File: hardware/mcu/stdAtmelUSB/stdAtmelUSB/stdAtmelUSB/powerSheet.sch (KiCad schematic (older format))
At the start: 22 parts, among them J1 Conn_01x03_Male, U1 LTC3406ES5, U2 MAX40200AUK, U3 LTC3406ES5, U4 MAX40200AUK

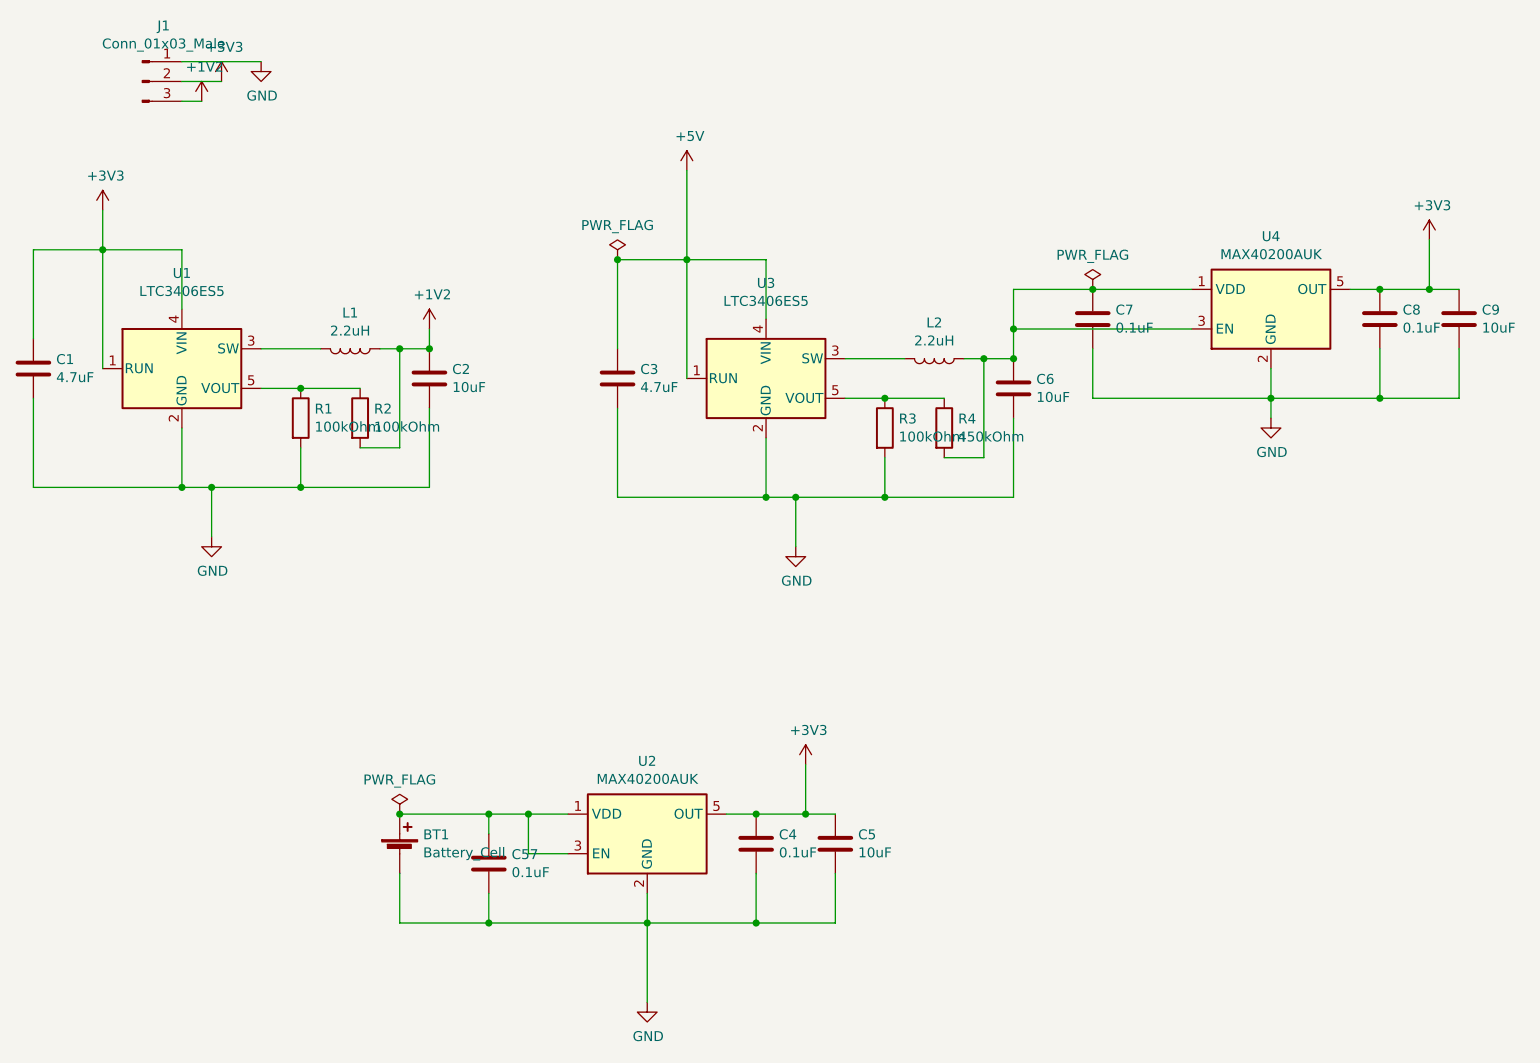
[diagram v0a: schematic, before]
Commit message: std MCU board
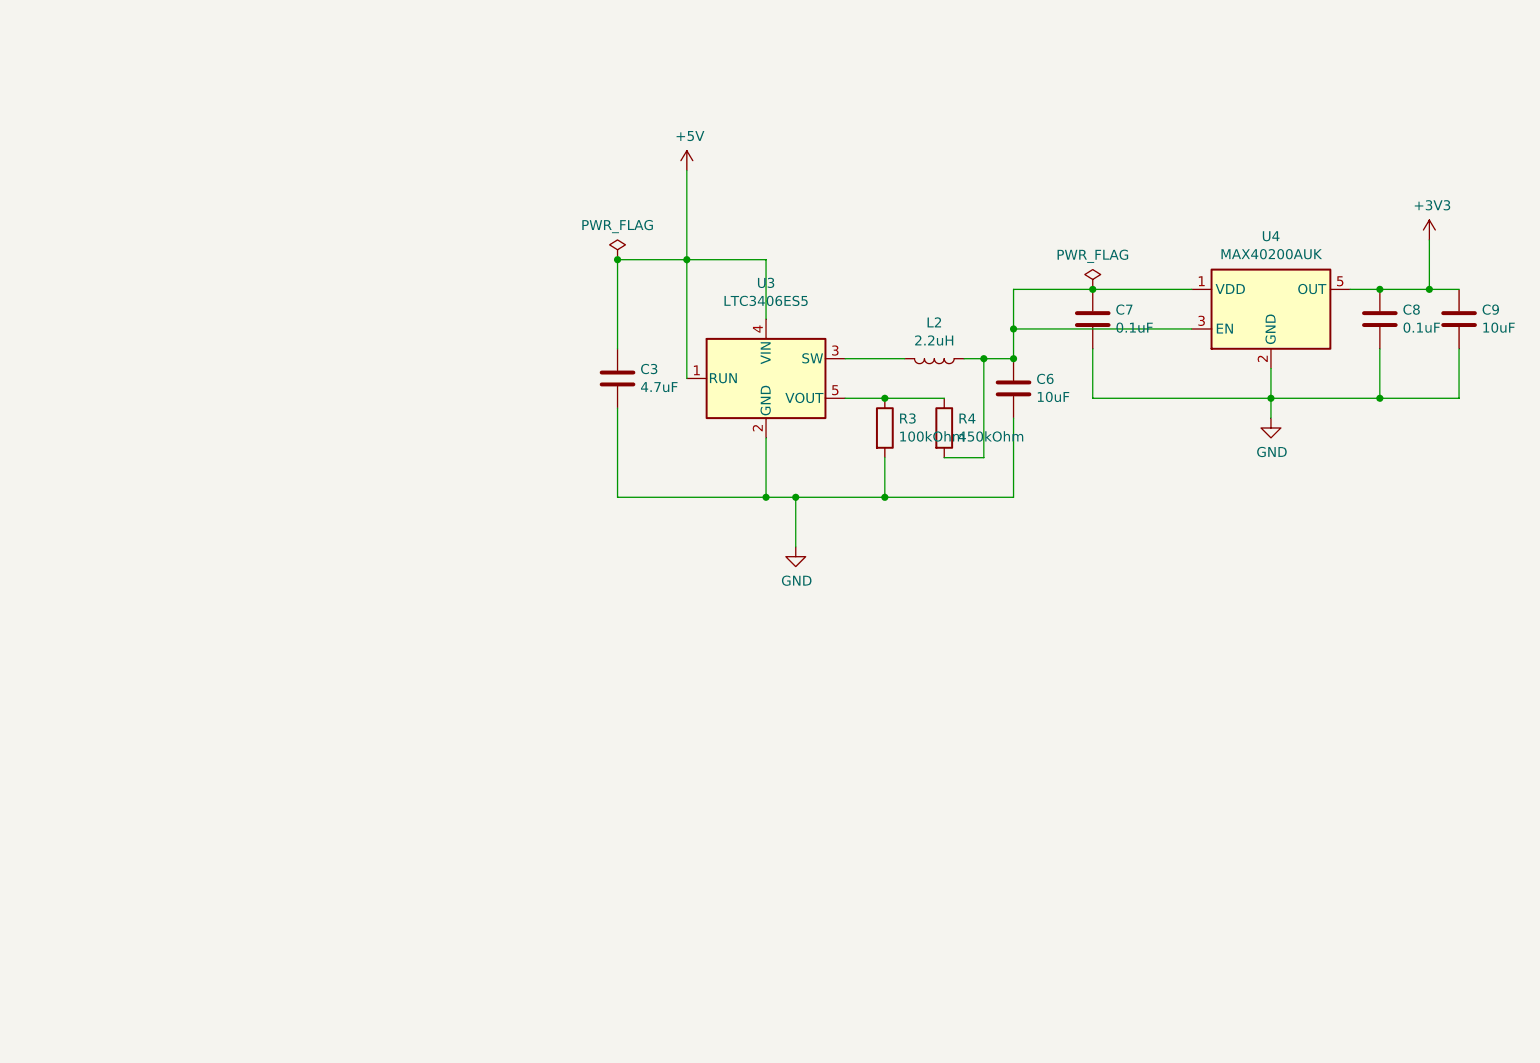
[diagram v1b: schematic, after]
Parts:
- removed BT1: Battery_Cell, kifootp:CR2032, symbol Device:Battery_Cell
- removed C1: 4.7uF, Capacitor_SMD:C_0402_1005Metric, symbol Device:C
- removed C2, C5: 10uF, Capacitor_SMD:C_0603_1608Metric, symbol Device:C
- removed C4, C57: 0.1uF, Capacitor_SMD:C_0402_1005Metric, symbol Device:C
- removed J1: Conn_01x03_Male, Connector_PinHeader_2.54mm:PinHeader_1x03_P2.54mm_Vertical, symbol Connector:Conn_01x03_Male
- removed L1: 2.2uH, Inductor_SMD:L_0805_2012Metric, symbol Device:L
- removed R1, R2: 100kOhm, Resistor_SMD:R_0402_1005Metric, symbol Device:R
- removed U1: LTC3406ES5, Package_TO_SOT_SMD:TSOT-23-5, symbol Regulator_Switching:LTC3406ES5
- removed U2: MAX40200AUK, Package_TO_SOT_SMD:SOT-23-5, symbol Analog_Switch:MAX40200AUK
